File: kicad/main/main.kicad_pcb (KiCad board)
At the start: 2 copper layers, 44.5 x 35 mm, 19 parts, among them J2 Conn_01x02, J3 Conn_01x07_Pin, J4 Conn_01x04_Pin, P1 USB_C_Plug_USB2.0, SW1 MK-12C03-G015, SW3 SW_Push, SW4 SW_Push, U1 HUSB237, U2 ZX-PH2.0-WT4P

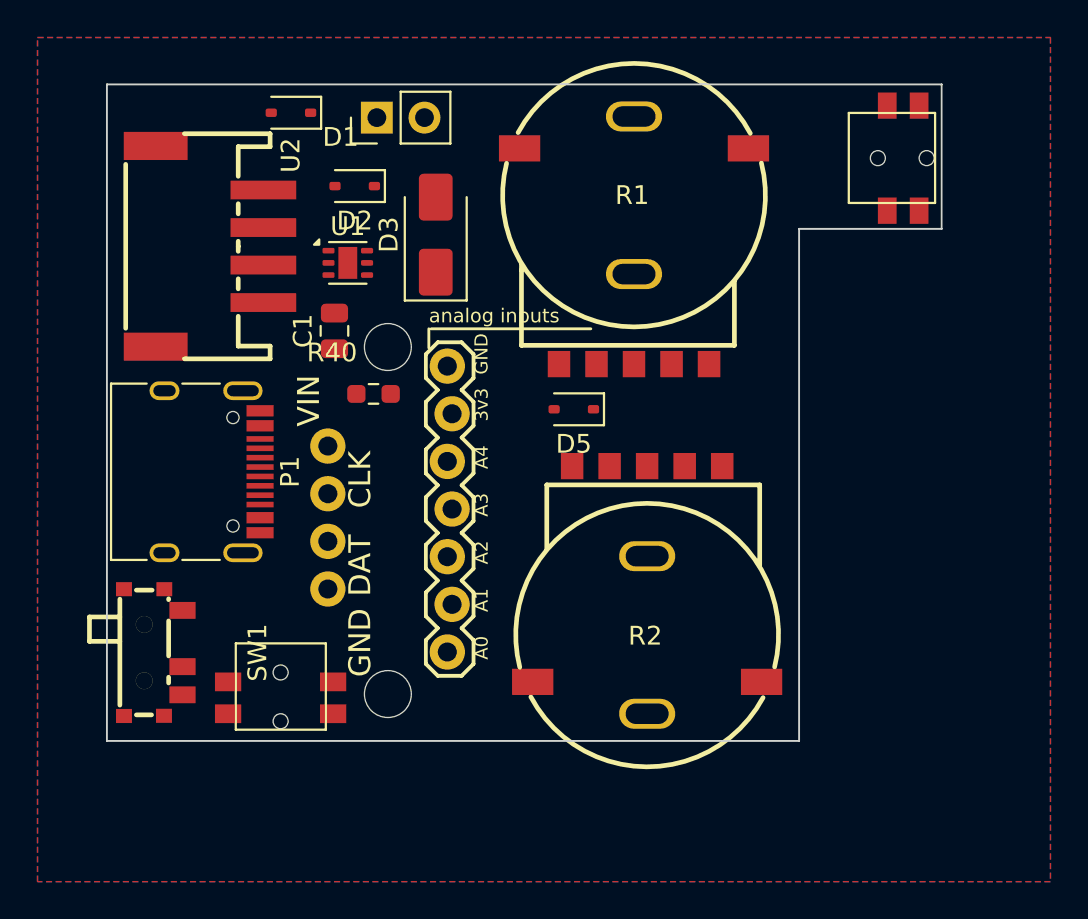
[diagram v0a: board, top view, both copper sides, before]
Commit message: Rewired PCB
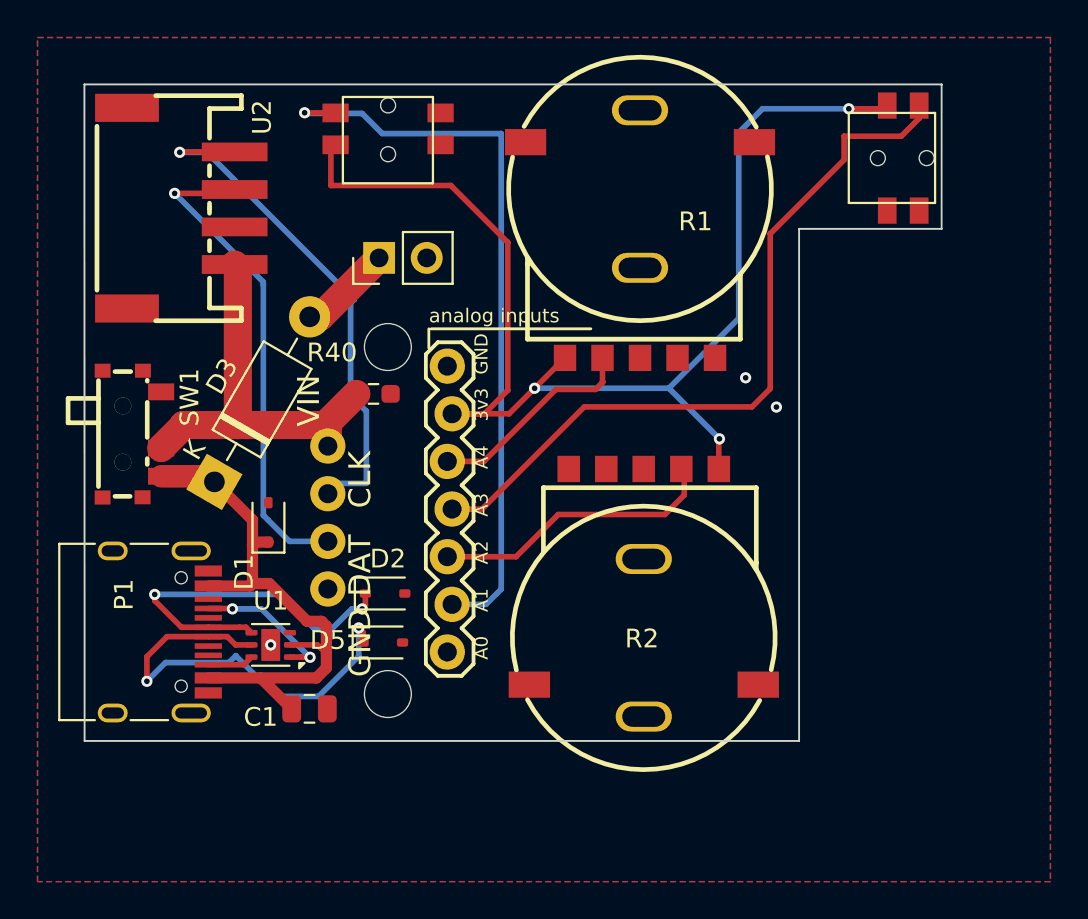
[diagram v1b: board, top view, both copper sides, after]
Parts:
- D3: value SS34 -> 1N4007; footprint Diode_SMD:D_SMA -> Diode_THT:D_DO-41_SOD81_P10.16mm_Horizontal
- moved SW3 30.8 mm to (176.2, 77.4), turned to 180 degrees
- moved D1 21.9 mm to (169.8, 98.3), turned to 90 degrees
- moved D2 21.8 mm to (176.0, 102.1), turned to 0 degrees
- moved U1 20.8 mm to (169.9, 104.9), turned to 180 degrees
- moved C1 20.2 mm to (172.0, 108.3), turned to 0 degrees
- moved D3 17.7 mm to (166.9, 96.2), turned to 60 degrees
- moved D5 16.1 mm to (175.9, 104.8), turned to 0 degrees
- moved SW1 11.7 mm to (162.5, 93.6)
- moved P1 8.97 mm to (162.6, 104.2)
- moved J2 7.48 mm to (175.7, 84.2)
- moved U2 2.54 mm to (165.1, 81.6)
- moved R1 0.46 mm to (189.6, 83.0)
- moved R2 0.23 mm to (189.8, 102.1)
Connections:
- D2 pad 1: GND -> D+
- D2 pad 2: D+ -> GND
- D5 pad 1: GND -> D-
- D5 pad 2: D- -> GND
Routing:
- net +3V3: track 0.00 -> 68.0 mm, vias 0 -> 3
- net AIN1: track 0.00 -> 39.9 mm, vias 0 -> 1
- net AIN3: track 0.00 -> 39.8 mm
- net VBUS: track 0.00 -> 30.6 mm
- net SCK_OUT: track 0.00 -> 28.0 mm, vias 0 -> 1
- net MOSI_OUT: track 0.00 -> 26.4 mm, vias 0 -> 1
- net D-: track 0.00 -> 23.6 mm, vias 0 -> 2
- net VIN: track 0.00 -> 22.5 mm
- net D+: track 0.00 -> 19.4 mm, vias 0 -> 2
- net AIN2: track 0.00 -> 15.5 mm
- net AIN4: track 0.00 -> 11.3 mm
- net CC1: track 0.00 -> 7.58 mm, vias 0 -> 2
- net Net-(D3-A): track 0.00 -> 5.00 mm
- net CC2: track 0.00 -> 2.47 mm
- net GND: vias 0 -> 3
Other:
- board size 44.5 x 35 mm -> 45.7 x 35 mm
